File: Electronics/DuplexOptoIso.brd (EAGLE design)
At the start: 36.5 x 21.6 mm, 9 parts

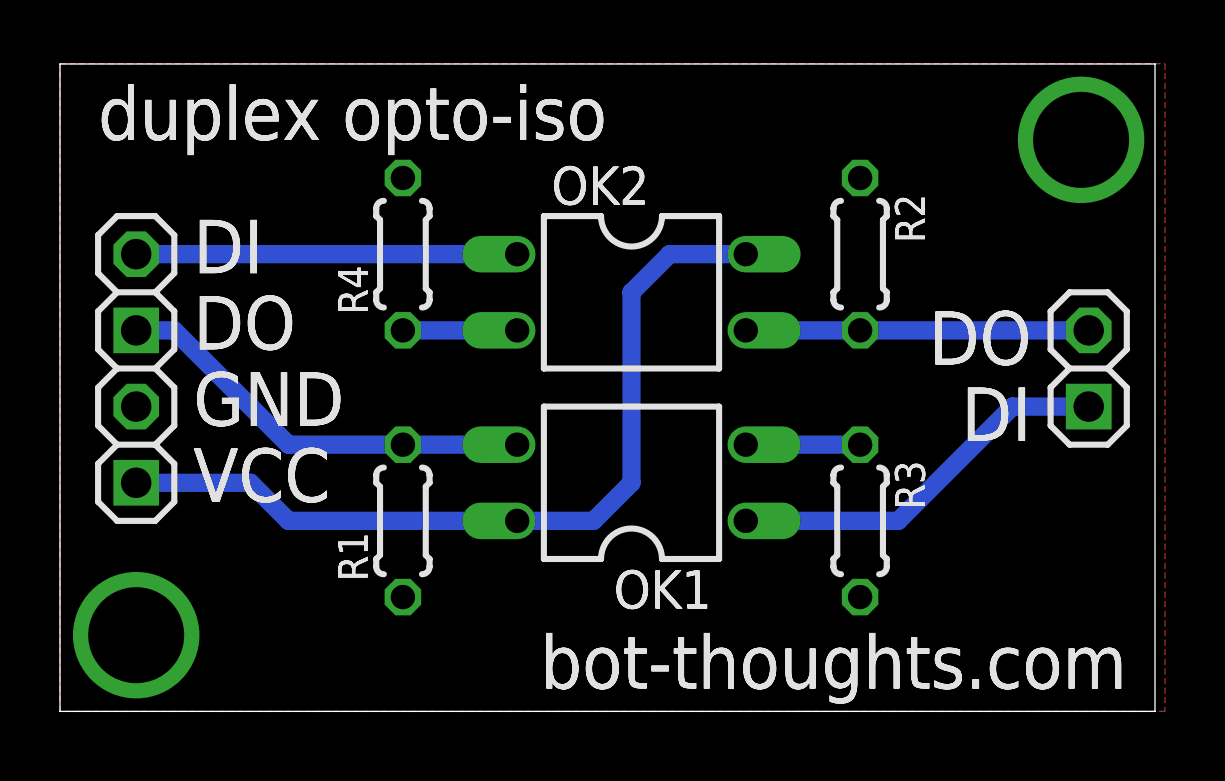
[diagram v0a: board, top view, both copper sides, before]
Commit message: Various tweaks
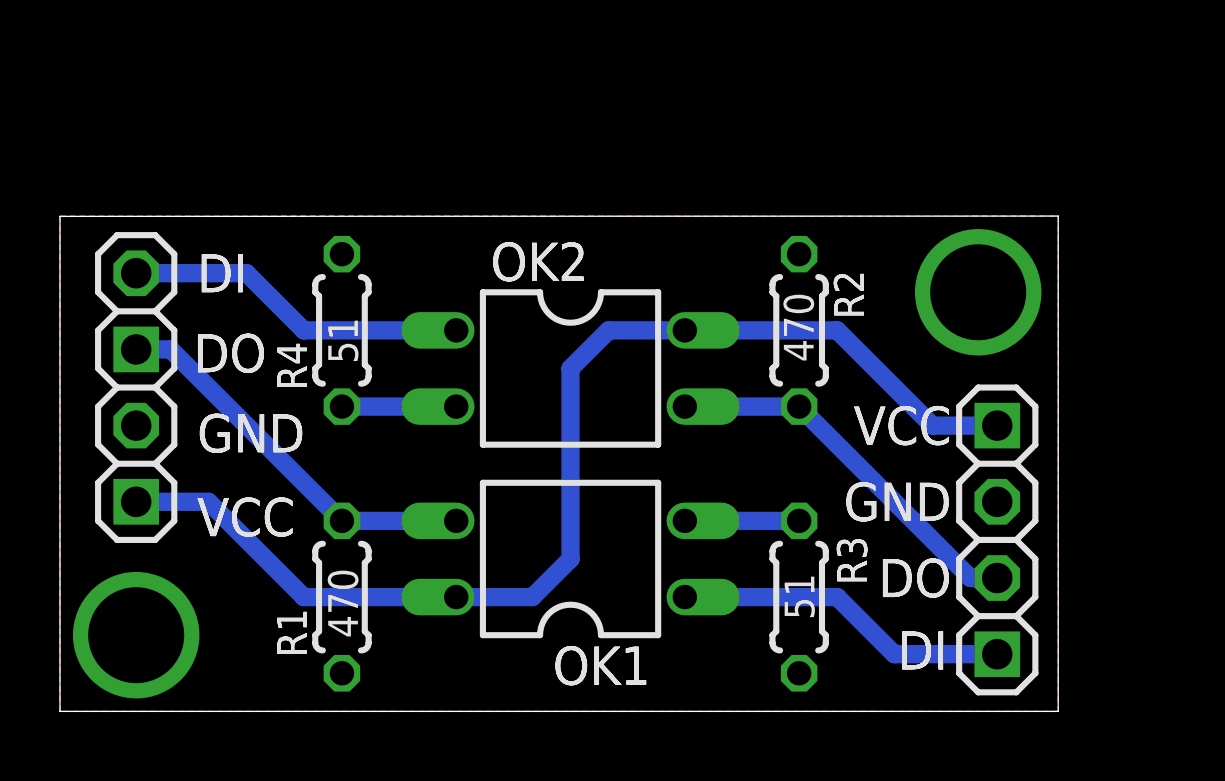
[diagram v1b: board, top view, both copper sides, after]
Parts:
- added JP4: POWER, pinhead-2:1X02-S
- R1, R2: value (none) -> 470
- R3, R4: value (none) -> 51
- moved JP1 8.80 mm to (31.2, 3.17)
- moved OK2 3.25 mm to (17.0, 11.4)
- moved R2 3.25 mm to (24.6, 12.7)
- moved R4 3.25 mm to (9.40, 12.7)
- moved OK1 3.25 mm to (17.0, 5.08)
- moved R1 3.25 mm to (9.40, 3.81)
- moved R3 3.25 mm to (24.6, 3.81)
- moved JP2 0.63 mm to (2.54, 13.3)
- moved JP3 0.63 mm to (2.54, 8.26)
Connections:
- net 5V: now also JP4.1
- net GND: now also JP4.2
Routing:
- net 5V: track 28.2 -> 38.7 mm
- net IN1: track 13.0 -> 11.2 mm
- net OUT2: track 11.4 -> 12.8 mm
- net IN2: track 12.7 -> 11.5 mm
- net OUT1: track 14.3 -> 13.0 mm
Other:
- board size 36.5 x 21.6 mm -> 33.3 x 16.5 mm
- board text added: "470"
- board text added: "51"
- board text added: "Rev 0.2"
